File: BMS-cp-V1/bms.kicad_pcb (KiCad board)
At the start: 2 copper layers, 60 x 40 mm, 8 parts

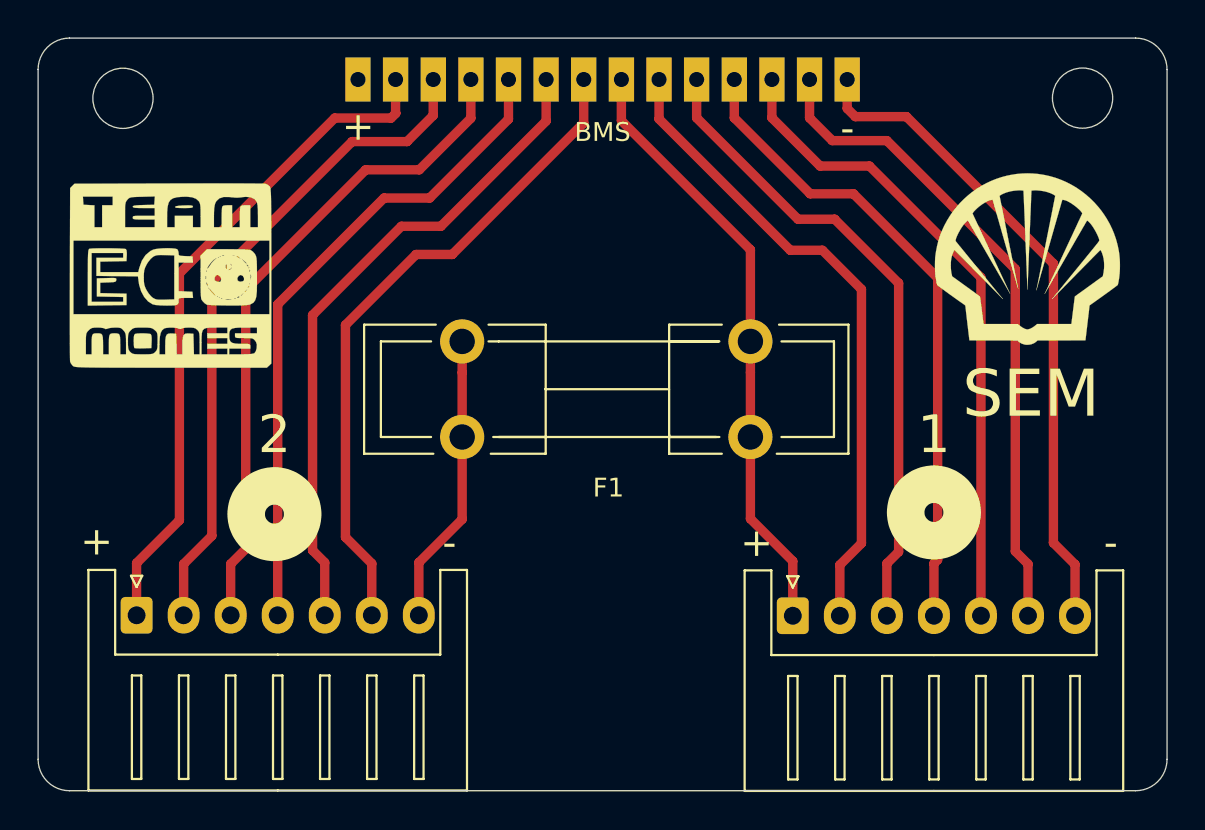
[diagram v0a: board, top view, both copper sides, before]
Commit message: Mise à jour prennant en compte les nouvelles cotes définies par Nicolas, le 17/02/2020.
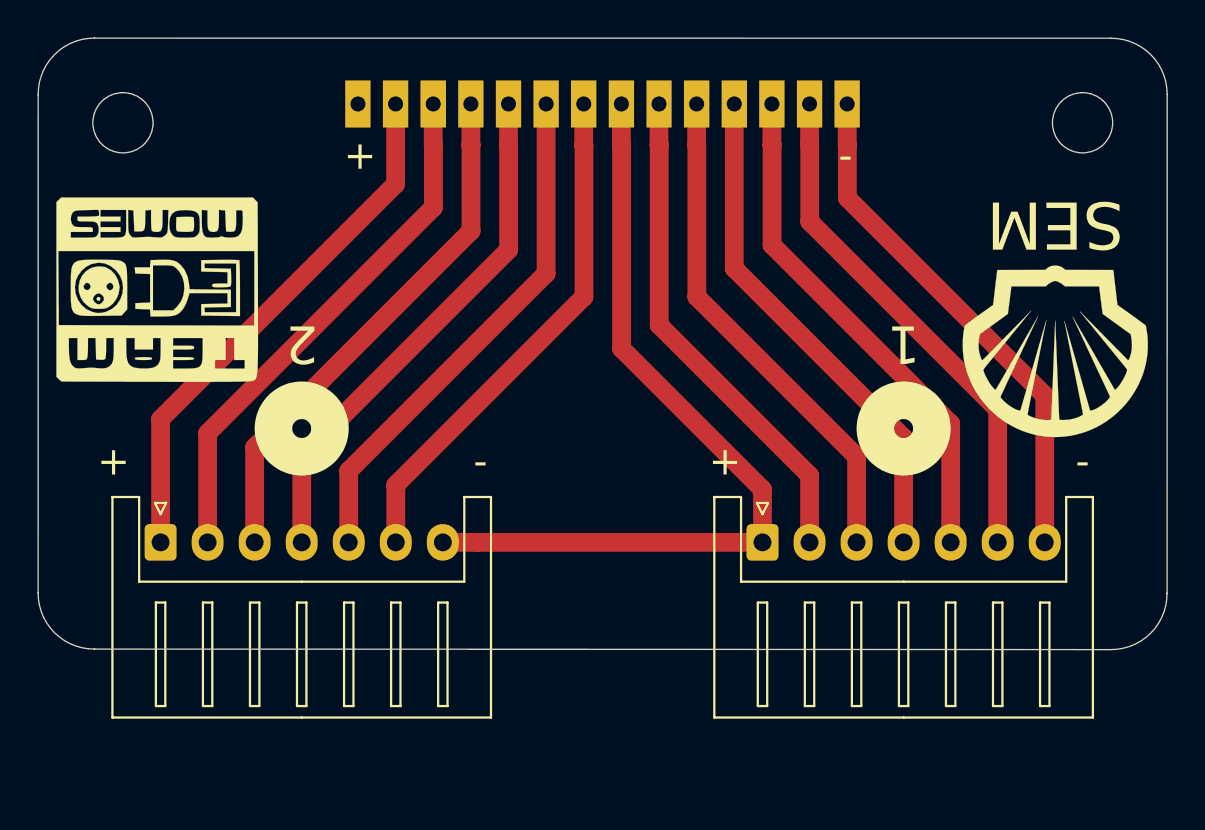
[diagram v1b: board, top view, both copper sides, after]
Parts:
- removed F1: Fuse, Fuse_Holders_and_Fuses:Fuseholder5x20_horiz_open_lateral_Type-II
- removed the G*** at (97.0, 92.6)
- removed the REF** at (145.5, 83.2)
- removed the REF** at (94.5, 83.2)
- added G***: LOGO, Symbol:logo-EcoMomes, F.Cu at (96.3, 93.4)
- added REF**: MountingHole_3.2mm_M3, MountingHole:MountingHole_3.2mm_M3, F.Cu at (145.5, 84.5)
- added REF**: MountingHole_3.2mm_M3, MountingHole:MountingHole_3.2mm_M3, F.Cu at (94.5, 84.5)
- moved G*** 5.13 mm to (144.1, 96.7), turned to 180 degrees
- moved -1+1 4.22 mm to (128.5, 106.8)
- moved -2+1 4.08 mm to (96.5, 106.8)
- moved BMS 1.30 mm to (133.0, 83.5)
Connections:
- -2+1 pad 7: Net-(-2+1-Pad7) -> Net-(-1+1-Pad1)
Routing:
- net Net-(-2+1-Pad7): track 15.5 -> 0.00 mm
- net Net-(-1+1-Pad1): track 32.3 -> 43.4 mm
- net Net-(-2+1-Pad6): track 35.4 -> 27.4 mm
- net Net-(-1+1-Pad2): track 34.4 -> 26.6 mm
- net Net-(-1+1-Pad6): track 35.0 -> 27.4 mm
- net Net-(-1+1-Pad3): track 34.3 -> 26.8 mm
- net Net-(-2+1-Pad5): track 35.1 -> 27.6 mm
- net Net-(-1+1-Pad7): track 35.1 -> 27.6 mm
- net Net-(-1+1-Pad5): track 34.6 -> 27.2 mm
- net Net-(-1+1-Pad4): track 34.4 -> 27.0 mm
- net Net-(-2+1-Pad3): track 35.4 -> 28.1 mm
- net Net-(-2+1-Pad1): track 35.8 -> 28.5 mm
- net Net-(-2+1-Pad2): track 35.5 -> 28.3 mm
- net Net-(-2+1-Pad4): track 35.1 -> 27.9 mm
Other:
- board size 60 x 40 mm -> 60 x 32.5 mm
